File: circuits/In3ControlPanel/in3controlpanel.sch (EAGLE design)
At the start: 24 parts, among them SW1 EC12E_SW

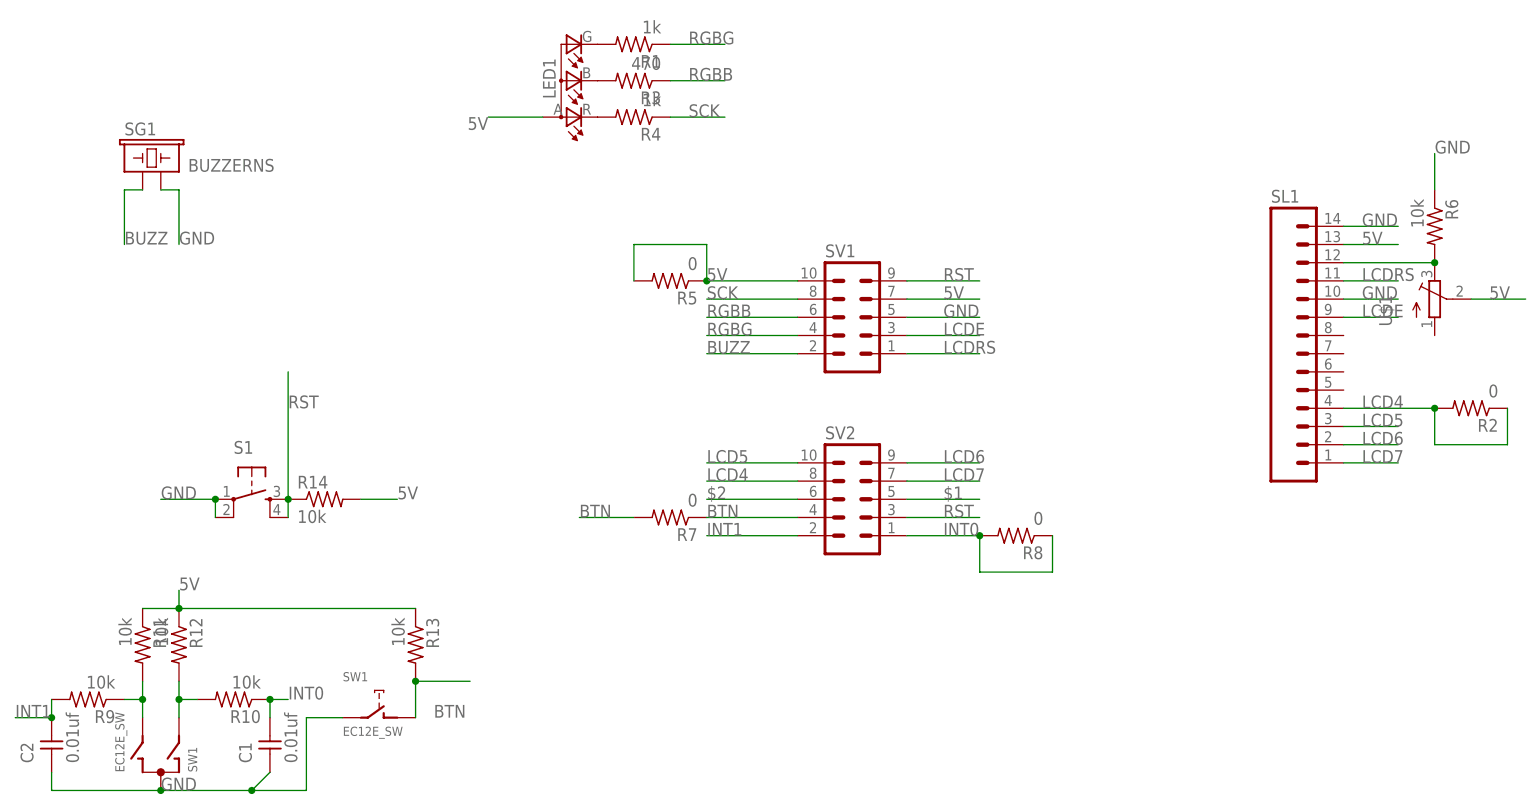
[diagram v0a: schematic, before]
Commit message: New Electronics
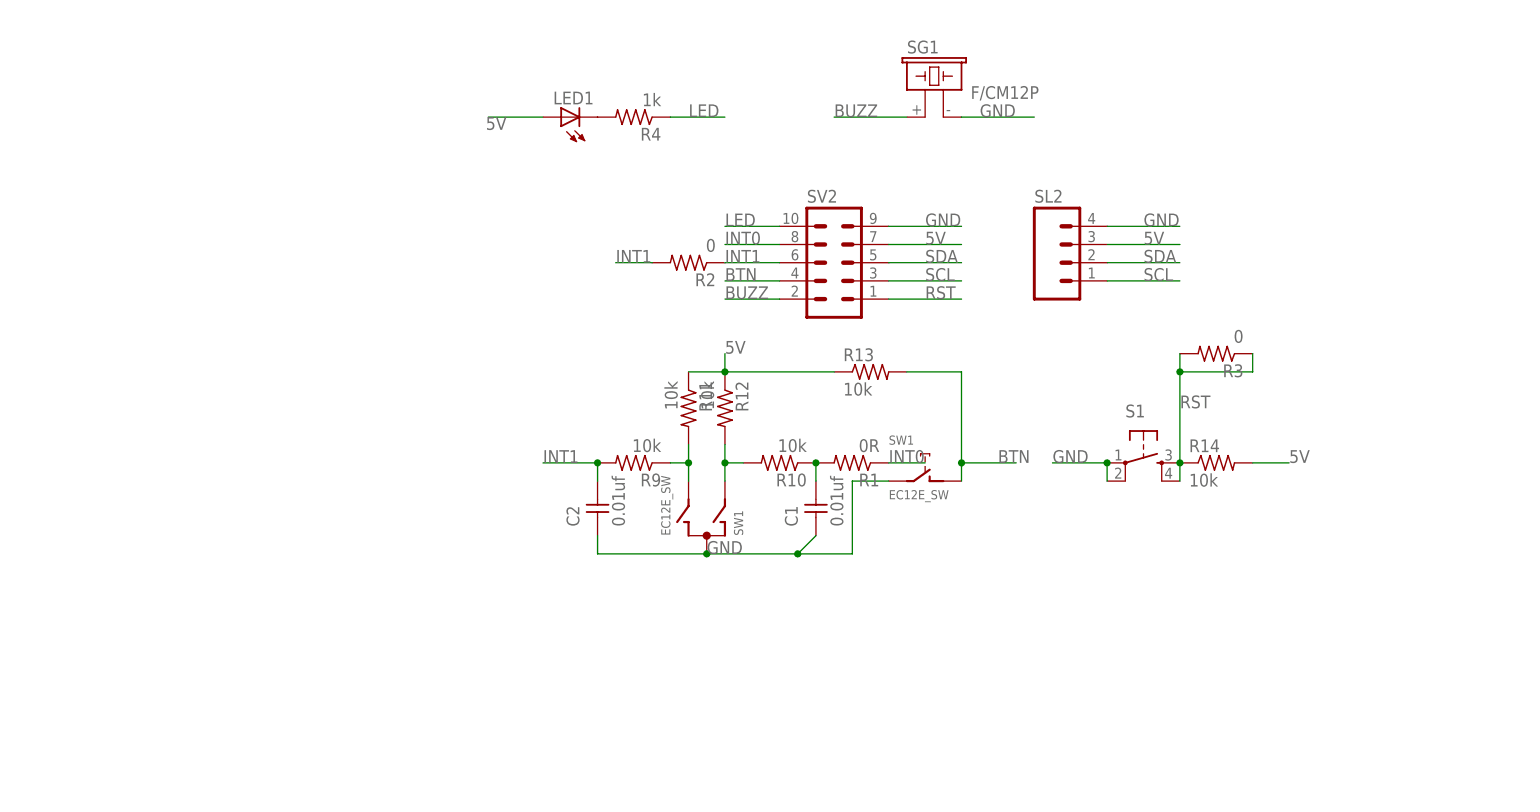
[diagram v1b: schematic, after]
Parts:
- removed R5, R7, R8: 0, ng:RESISTOR1206
- removed R6: 10k, ng:RESISTOR1206
- removed SL1: (no value), con-amp-quick:MA14
- removed SV1: (no value), con-lstb:MA05-2
- removed U$1: (no value), 01_adafruit:TRIMPOTTC33X
- added SL2: (no value), con-amp-quick:MA04
- LED1: device 01_fab:LEDRGBOLD -> eagle-ltspice:LED_E
- R1: value 1k -> 0R
- R3: value 470 -> 0
- SG1: value BUZZERNS -> F/CM12P; device 01_SparkFun:BUZZERNS -> buzzer:F/CM12P
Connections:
- removed net $1: SV2.5
- removed net $2: SV2.6
- removed net LCD4: R2.1, R2.2, SL1.4, SV2.8
- removed net LCD5: SL1.3, SV2.10
- removed net LCD6: SL1.2, SV2.9
- removed net LCD7: SL1.1, SV2.7
- removed net LCDE: SL1.9, SV1.3
- removed net LCDRS: SL1.11, SV1.1
- removed net N$2: LED1.CGREEN, R1.2
- removed net N$3: LED1.CBLUE, R3.2
- removed net N$4: LED1.CRED, R4.2
- removed net N$6: R6.2, SL1.12, U$1.E
- removed net RGBB: R3.1, SV1.6
- removed net RGBG: R1.1, SV1.4
- removed net SCK: R4.1, SV1.8
- new net LED: R4.1, SV2.10
- new net N$1: LED1.C, R4.2
- new net SCL: SL2.1, SV2.3
- new net SDA: SL2.2, SV2.5
- net 5V: now also LED1.A, SL2.3, SV2.7; no longer LED1.A2, R5.1, R5.2, SL1.13, SV1.10, SV1.7, U$1.S
- net BTN: no longer R7.1, R7.2
- net BUZZ: now also SV2.2; no longer SV1.2
- net GND: now also SL2.4, SV2.9; no longer R6.1, SL1.10, SL1.14, SV1.5
- net INT0: now also R1.1, R1.2, SV2.8; no longer R8.1, R8.2, SV2.1
- net INT1: now also R2.1, R2.2, SV2.6; no longer SV2.2
- net RST: now also R3.1, R3.2, SV2.1; no longer SV1.9, SV2.3
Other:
- moved on the sheet: C1, C2, R1, R10, R11, R12, R13, R14, R2, R3, R9, S1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
